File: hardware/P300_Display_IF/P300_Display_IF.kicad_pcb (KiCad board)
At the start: 2 copper layers, 6 parts, among them J15 TFT Display 1, J16 TFT Display 2

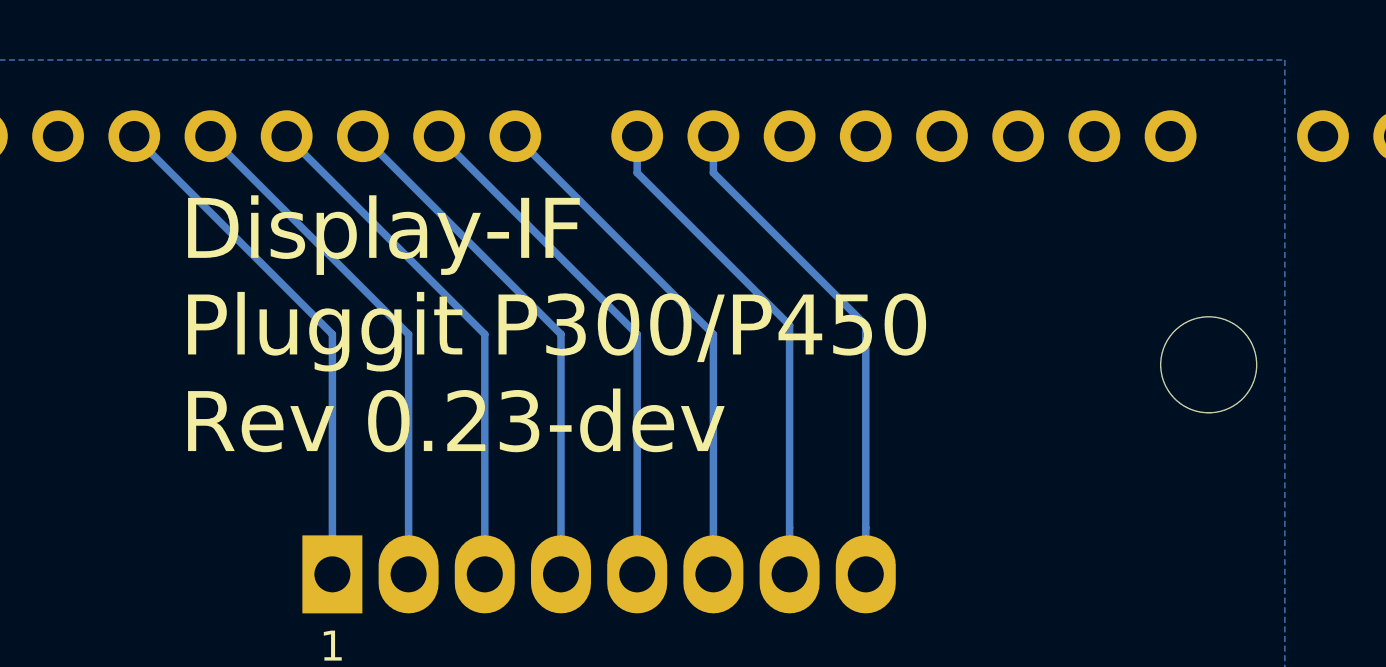
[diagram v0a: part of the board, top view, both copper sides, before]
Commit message: Platinen V.23 in die Herstellung gegeben
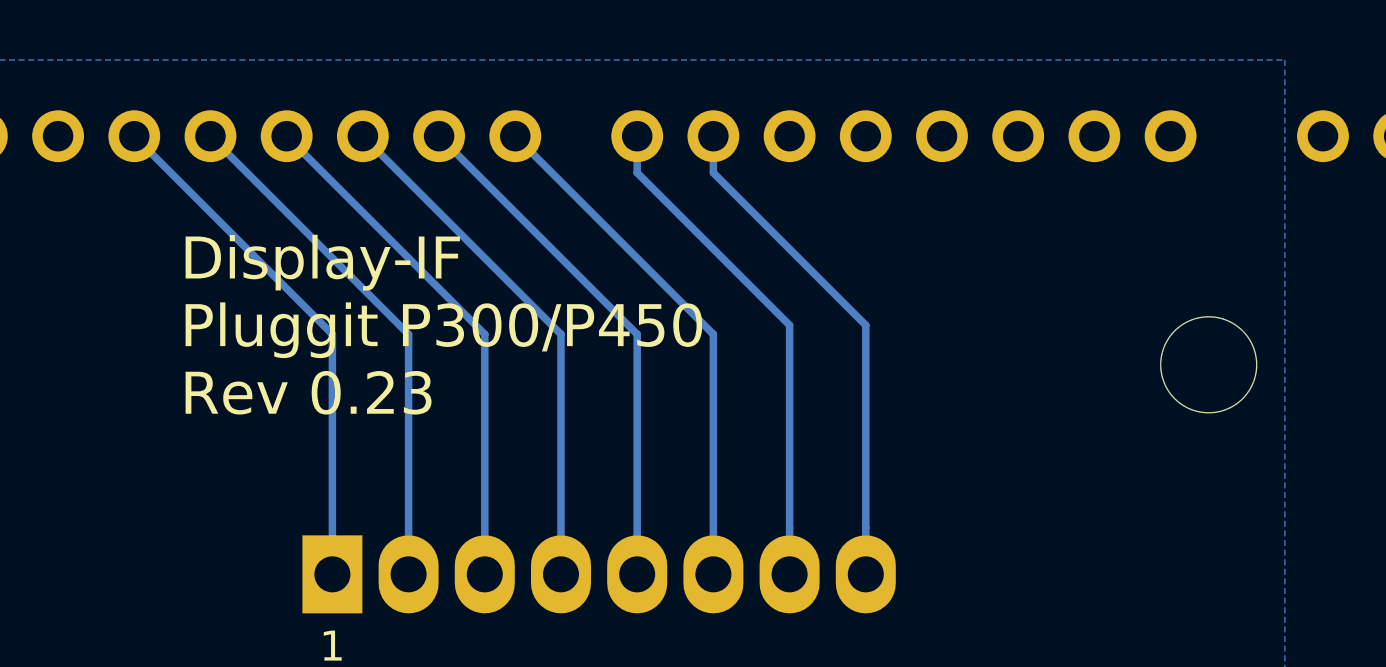
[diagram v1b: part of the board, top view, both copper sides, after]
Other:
- board text added: "Display-IF Pluggit P300/P450 Rev 0.23"
- board text removed: "Display-IF Pluggit P300/P450 Rev 0.23-dev"
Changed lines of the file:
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@@
-(kicad_pcb (version 20171130) (host pcbnew "(5.0.2)-1")
+(kicad_pcb (version 20171130) (host pcbnew "(5.0.1)-3")
   (general
     (thickness 1.6)
@@
     (effects (font (size 1 1) (thickness 0.25)) (justify left))
   )
-  (gr_text "Display-IF\nPluggit P300/P450\nRev 0.23-dev" (at 106.68 77.47) (layer F.SilkS)
-    (effects (font (size 2 2) (thickness 0.3)) (justify left))
+  (gr_text "Display-IF\nPluggit P300/P450\nRev 0.23" (at 106.68 77.47) (layer F.SilkS)
+    (effects (font (size 1.4 1.4) (thickness 0.2)) (justify left))
   )
   (dimension 53.34 (width 0.3) (layer F.Fab)
